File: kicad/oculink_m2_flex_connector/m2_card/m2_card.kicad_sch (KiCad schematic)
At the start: 14 parts, among them J1 G14A42121B12HR

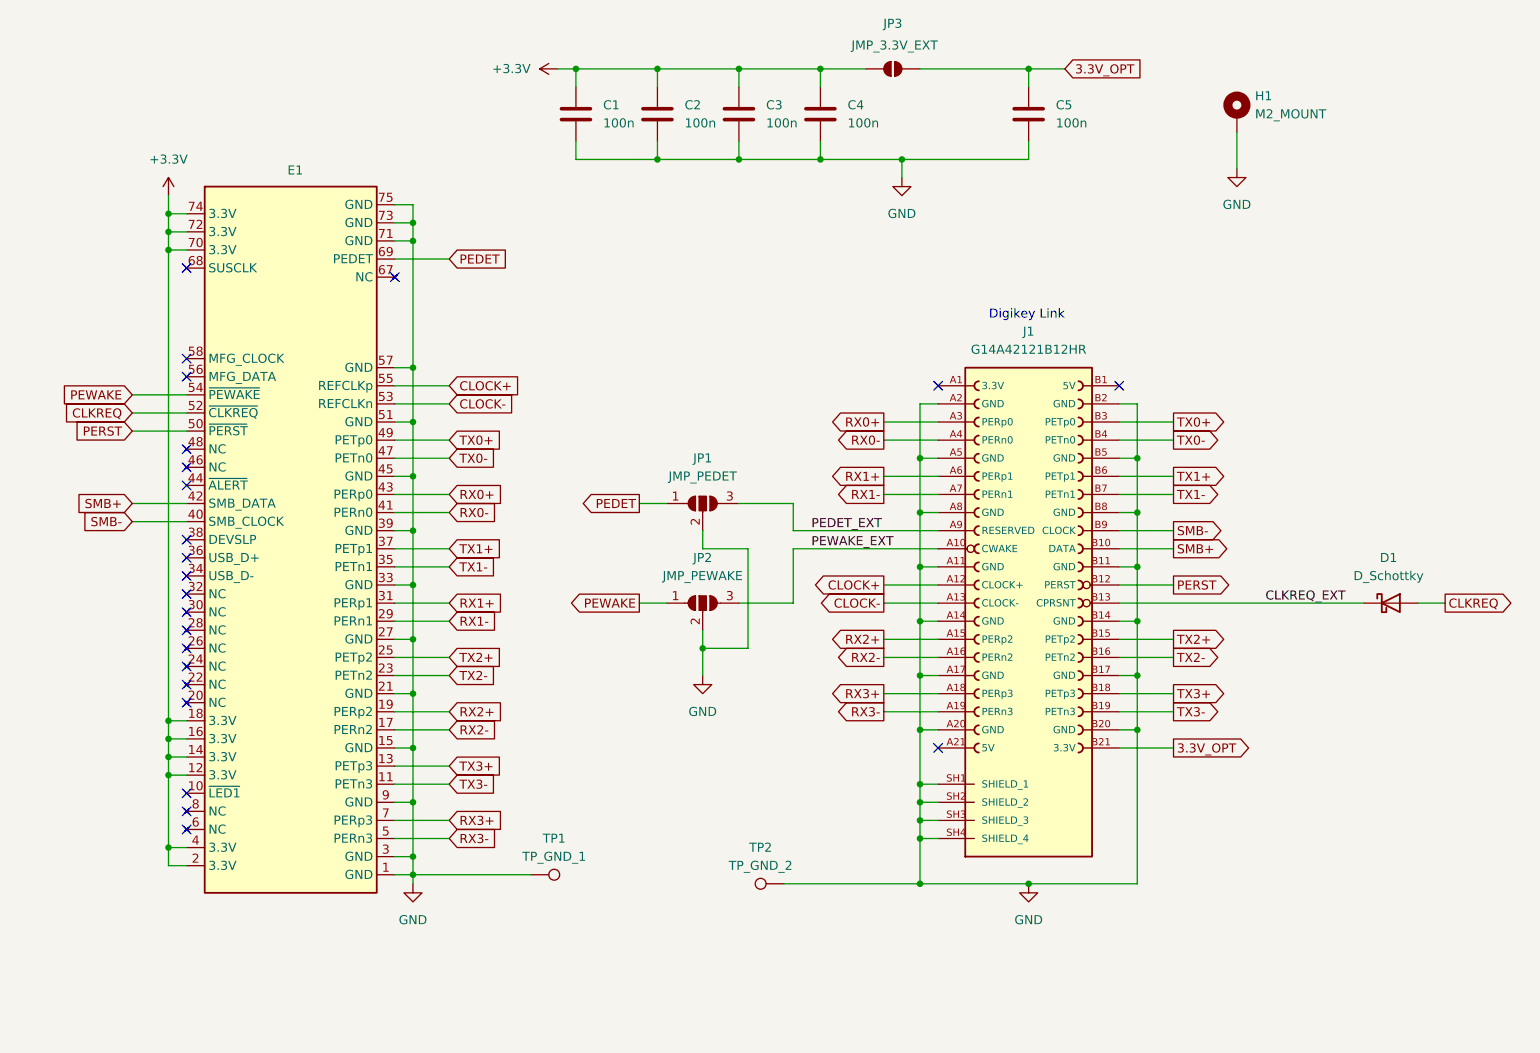
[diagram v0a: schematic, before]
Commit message: Finished first draft of m2 card
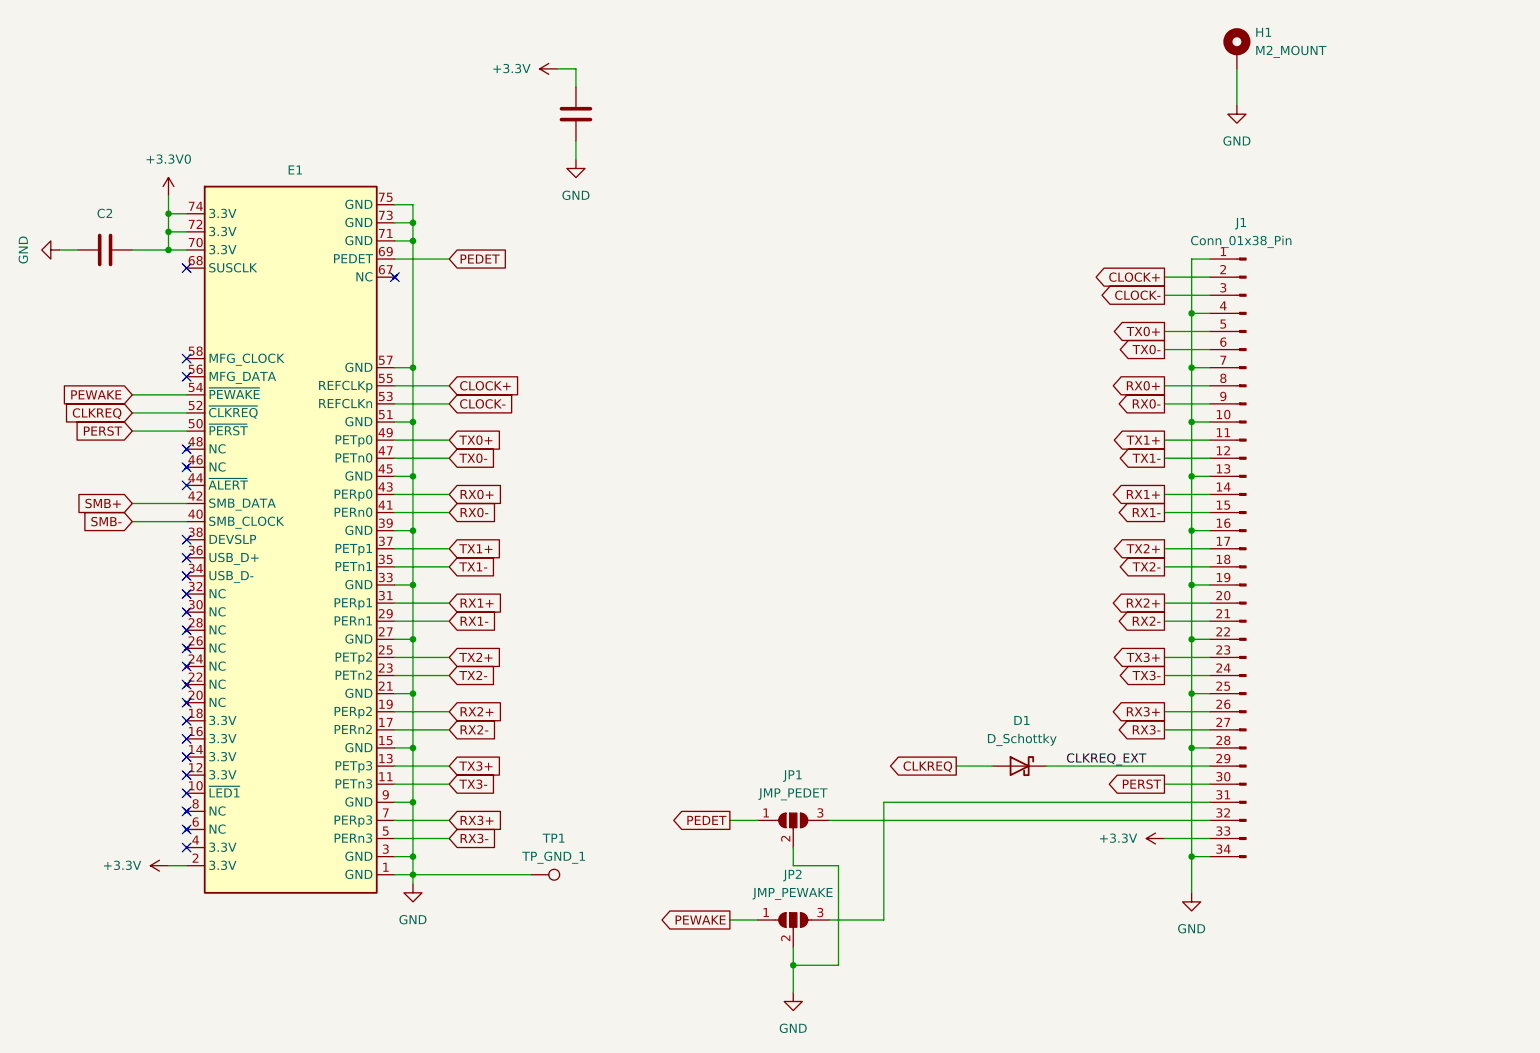
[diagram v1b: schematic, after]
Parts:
- removed C3, C4, C5: 100n, Capacitor_SMD:C_0402_1005Metric, symbol Device:C
- removed J1: G14A42121B12HR, amphenol_oculink:AMPHENOL_G14A42121B12HR, symbol G14A42121B12HR:G14A42121B12HR
- removed JP3: JMP_3.3V_EXT, Jumper:SolderJumper-2_P1.3mm_Open_RoundedPad1.0x1.5mm, symbol Jumper:SolderJumper_2_Open
- removed TP2: TP_GND_2, TestPoint:TestPoint_Pad_D1.0mm, symbol Connector:TestPoint
- added J1: Conn_01x38_Pin, flex_connector:port_pcb, symbol Connector:Conn_01x34_Pin
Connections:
- net +3.3V: now also J1.33 (Pin_33); no longer C2.1, E1.12 (3.3V), E1.14 (3.3V), E1.16 (3.3V), E1.18 (3.3V), E1.4 (3.3V), E1.70 (3.3V), E1.72 (3.3V), E1.74 (3.3V)
- net CLKREQ_EXT: now also J1.29 (Pin_29)
- net CLOCK+: now also J1.2 (Pin_2)
- net CLOCK-: now also J1.3 (Pin_3)
- net GND: now also C2.1, J1.1 (Pin_1), J1.10 (Pin_10), J1.13 (Pin_13), J1.16 (Pin_16), J1.19 (Pin_19), J1.22 (Pin_22), J1.25 (Pin_25), J1.28 (Pin_28), J1.34 (Pin_34), J1.4 (Pin_4), J1.7 (Pin_7); no longer C2.2
- net PERST: now also J1.30 (Pin_30)
- net RX0+: now also J1.8 (Pin_8)
- net RX0-: now also J1.9 (Pin_9)
- net RX1+: now also J1.14 (Pin_14)
- net RX1-: now also J1.15 (Pin_15)
- net RX2+: now also J1.20 (Pin_20)
- net RX2-: now also J1.21 (Pin_21)
- net RX3+: now also J1.26 (Pin_26)
- net RX3-: now also J1.27 (Pin_27)
- net TX0+: now also J1.5 (Pin_5)
- net TX0-: now also J1.6 (Pin_6)
- net TX1+: now also J1.11 (Pin_11)
- net TX1-: now also J1.12 (Pin_12)
- net TX2+: now also J1.17 (Pin_17)
- net TX2-: now also J1.18 (Pin_18)
- net TX3+: now also J1.23 (Pin_23)
- net TX3-: now also J1.24 (Pin_24)
- net PEDET_EXT: no longer names the net of JP1.3 (B)
- net PEDET_EXT: now also J1.32 (Pin_32)
- net PEWAKE_EXT: no longer names the net of JP2.3 (B)
- net PEWAKE_EXT: now also J1.31 (Pin_31)
- new net +3.3V0: C2.2, E1.70 (3.3V), E1.72 (3.3V), E1.74 (3.3V)
- no-connect marks 23 -> 25
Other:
- note removed: "Digikey Link"
- moved on the sheet: D1, H1, JP1, JP2
